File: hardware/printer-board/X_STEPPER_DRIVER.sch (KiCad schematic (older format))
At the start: 9 parts, among them J3 MS_SELECT, J4 X, U3 A4988_MODULE

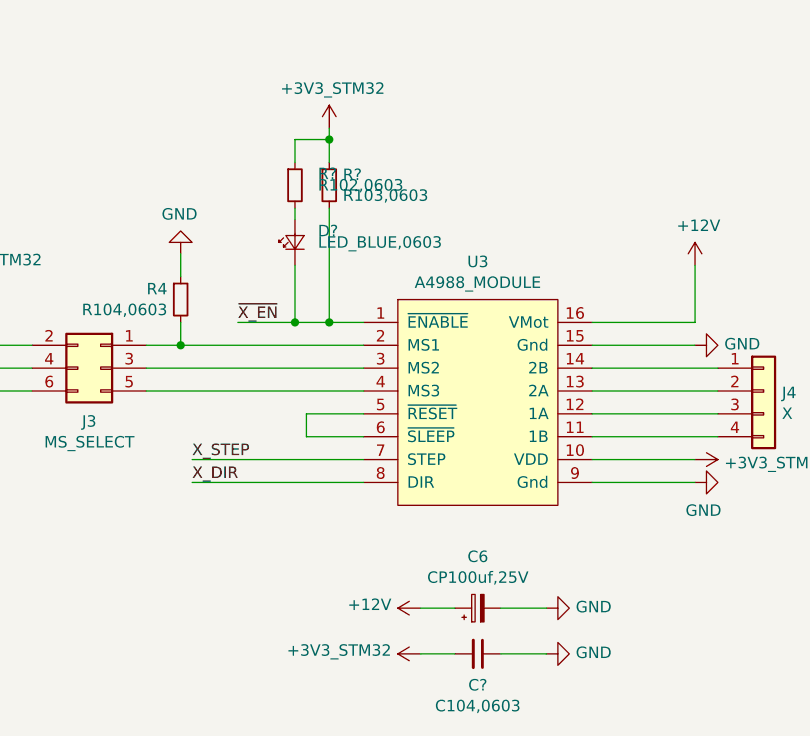
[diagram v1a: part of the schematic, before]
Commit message: update annotations,
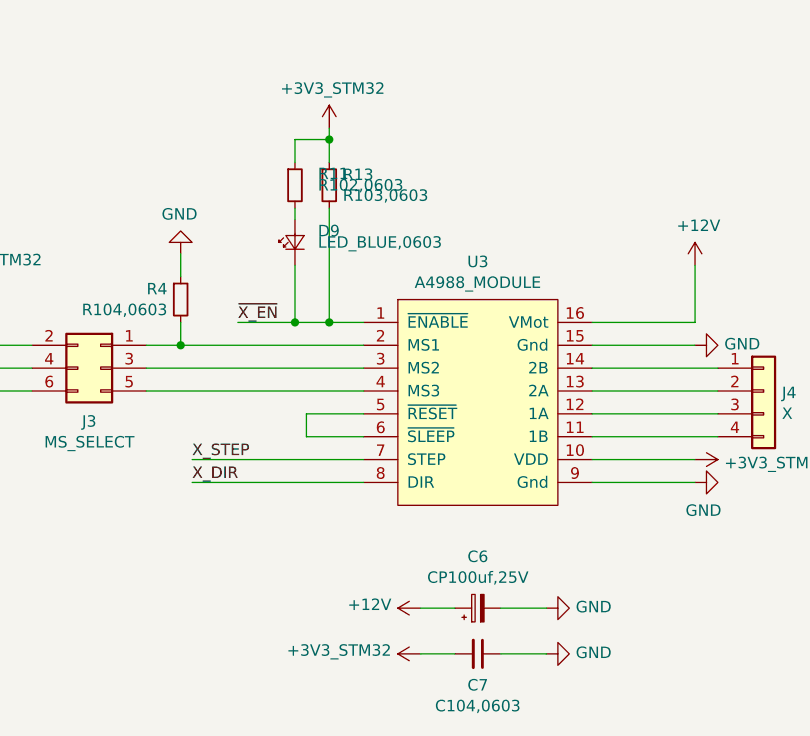
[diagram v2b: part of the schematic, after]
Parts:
- gave numbers to parts that had none: 4
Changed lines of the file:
@@
 $EndBitmap
 $Comp
-L taobao-components:+3V3_STM32 #PWR?
+L taobao-components:+3V3_STM32 #PWR011
 U 1 1 5CC40AA6
 P 3500 2700
-F 0 "#PWR?" H 3500 2550 50  0001 C CNN
+F 0 "#PWR011" H 3500 2550 50  0001 C CNN
 F 1 "+3V3_STM32" H 3515 2873 50  0000 C CNN
 F 2 "" H 3500 2700 50  0001 C CNN
@@
 $EndComp
 $Comp
-L taobao-components:+3V3_STM32 #PWR?
+L taobao-components:+3V3_STM32 #PWR013
 U 1 1 5CC40ABF
 P 5400 4250
-F 0 "#PWR?" H 5400 4100 50  0001 C CNN
+F 0 "#PWR013" H 5400 4100 50  0001 C CNN
 F 1 "+3V3_STM32" V 5415 4378 50  0000 L CNN
 F 2 "" H 5400 4250 50  0001 C CNN
@@
 $EndComp
 $Comp
-L taobao-components:+3V3_STM32 #PWR?
+L taobao-components:+3V3_STM32 #PWR012
 U 1 1 5CC40AED
 P 6600 3400
-F 0 "#PWR?" H 6600 3250 50  0001 C CNN
+F 0 "#PWR012" H 6600 3250 50  0001 C CNN
 F 1 "+3V3_STM32" V 6615 3528 50  0000 L CNN
 F 2 "" H 6600 3400 50  0001 C CNN
@@
 $EndComp
 $Comp
-L taobao-c:C104,0603 C?
+L taobao-c:C104,0603 C7
 U 1 1 5CC40BEE
 P 5650 4250
-F 0 "C?" V 5787 4250 50  0000 C CNN
+F 0 "C7" V 5787 4250 50  0000 C CNN
 F 1 "C104,0603" V 5878 4250 50  0000 C CNN
 F 2 "Capacitor_SMD:C_0603_1608Metric_Pad1.05x0.95mm_HandSolder" H 5650 4250 50  0001 C CNN
@@
 	4600 2800 4850 2800
 $Comp
-L taobao-r:R103,0603 R?
+L taobao-r:R103,0603 R13
 U 1 1 5CC5E2CE
 P 5000 2200
-AR Path="/5CC02AB8/5CC5E2CE" Ref="R?"  Part="1"
+AR Path="/5CC02AB8/5CC5E2CE" Ref="R13"  Part="1"
 AR Path="/5CC049BB/5CC5E2CE" Ref="R?"  Part="1"
 AR Path="/5CC0A4B9/5CC5E2CE" Ref="R?"  Part="1"
@@
 AR Path="/5CC0A8CF/5CC5E2CE" Ref="R?"  Part="1"
 AR Path="/5CC0AEC9/5CC5E2CE" Ref="R?"  Part="1"
-F 0 "R?" H 5059 2246 50  0000 L CNN
+F 0 "R13" H 5059 2246 50  0000 L CNN
 F 1 "R103,0603" H 5059 2155 50  0000 L CNN
 F 2 "Resistor_SMD:R_0603_1608Metric_Pad1.05x0.95mm_HandSolder" H 5000 2200 50  0001 C CNN
@@
 P 5000 1950
 AR Path="/5CC0AEC9/5CC5E2D6" Ref="#PWR?"  Part="1"
-AR Path="/5CC02AB8/5CC5E2D6" Ref="#PWR?"  Part="1"
-F 0 "#PWR?" H 5000 1800 50  0001 C CNN
+AR Path="/5CC02AB8/5CC5E2D6" Ref="#PWR010"  Part="1"
+F 0 "#PWR010" H 5000 1800 50  0001 C CNN
 F 1 "+3V3_STM32" H 5015 2123 50  0000 C CNN
 F 2 "" H 5000 1950 50  0001 C CNN
@@
 AR Path="/5CC15C35/5CC5E2DC" Ref="R?"  Part="1"
 AR Path="/5CC0AEC9/5CC5E2DC" Ref="R?"  Part="1"
-AR Path="/5CC02AB8/5CC5E2DC" Ref="R?"  Part="1"
-F 0 "R?" H 4950 2250 50  0000 L CNN
+AR Path="/5CC02AB8/5CC5E2DC" Ref="R11"  Part="1"
+F 0 "R11" H 4950 2250 50  0000 L CNN
 F 1 "R102,0603" H 4950 2200 50  0000 L CNN
 F 2 "Resistor_SMD:R_0603_1608Metric_Pad1.05x0.95mm_HandSolder" H 4850 2200 50  0001 C CNN
@@
 AR Path="/5CC15C35/5CC5E2E3" Ref="D?"  Part="1"
 AR Path="/5CC0AEC9/5CC5E2E3" Ref="D?"  Part="1"
-AR Path="/5CC02AB8/5CC5E2E3" Ref="D?"  Part="1"
-F 0 "D?" V 4900 2350 50  0000 R CNN
+AR Path="/5CC02AB8/5CC5E2E3" Ref="D9"  Part="1"
+F 0 "D9" V 4900 2350 50  0000 R CNN
 F 1 "LED_BLUE,0603" V 4850 2350 50  0000 R CNN
 F 2 "LED_SMD:LED_0603_1608Metric_Pad1.05x0.95mm_HandSolder" V 4850 2450 50  0001 C CNN
